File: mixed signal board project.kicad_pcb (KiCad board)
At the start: 4 copper layers, 70.4 x 72.2 mm, 189 parts, among them J101 USB_B_Mini, J102 Conn_01x06_Pin, J201 8P8C_Shielded, J301 Conn_01x04_Pin, J401 AudioJack2_Ground, J402 Conn_01x04_Pin, J403 Screw_Terminal_01x03, J501 USB_B_Mini, J701 Conn_01x02_Socket, J801 Conn_01x02_Socket, J901 UART_CONN, J902 CAN_CONN, SW101 SW_SPDT, SW201 SW_SPDT, SW901 SW_SPDT, U101 STM32F103C8Tx, U11 LD1117S33TR_SOT223, U12 LD1117S18TR_SOT223, U201 DP83826ERHBR, U301 ADS122C04IPW, U401 CS43L22-CNZ, U402 IMP34DT05TR, U501 CH340C, U701 DMHT6016LFJ-13, U702 DRV8701, U801 DMHT6016LFJ-13, U802 DRV8701, U901 STM32F407VGTx, Y201 25Mhz, Y901 8MHz

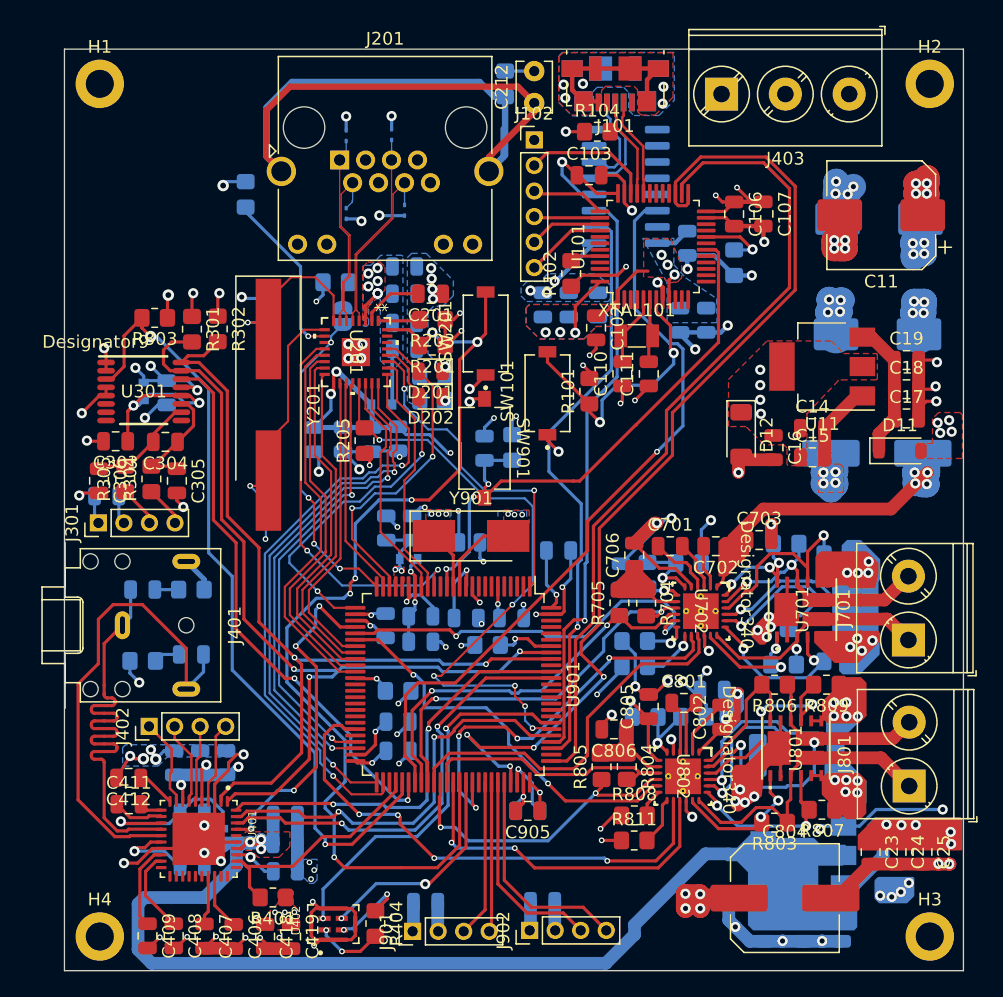
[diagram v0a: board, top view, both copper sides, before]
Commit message: schematic pages are reviewed
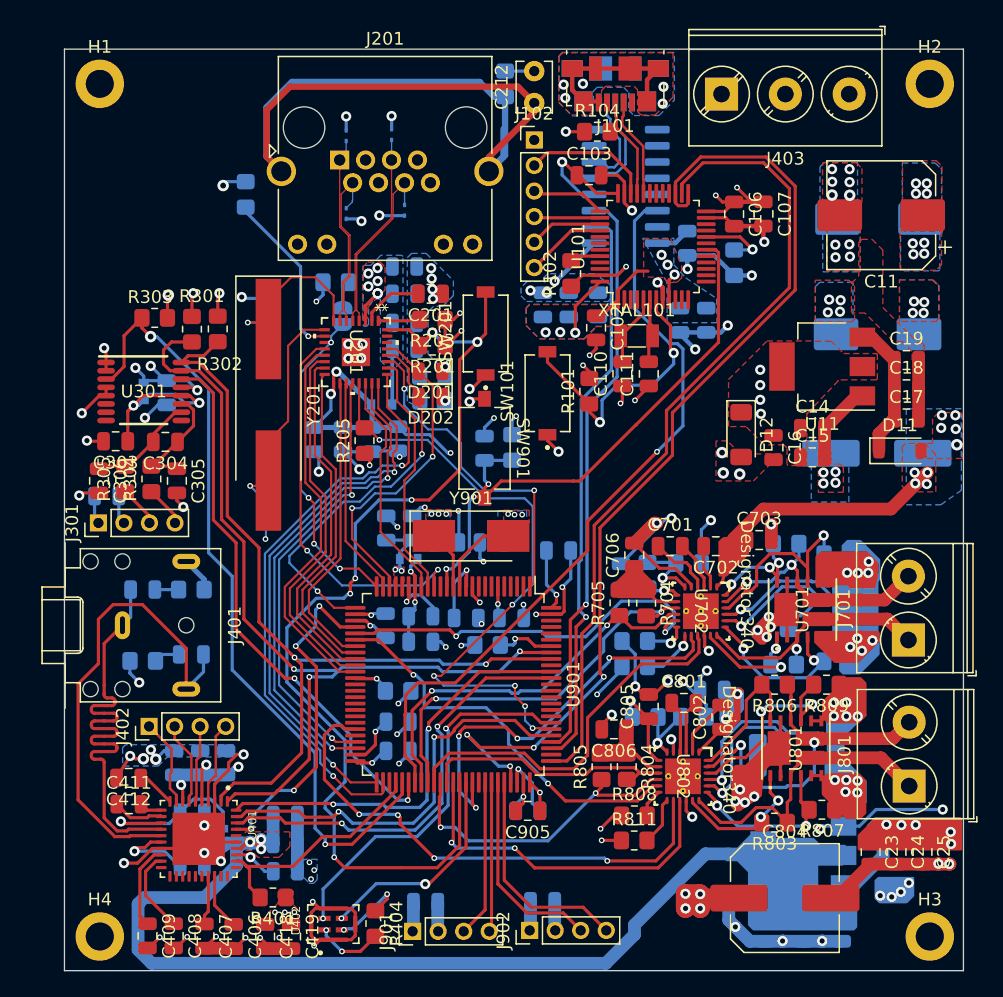
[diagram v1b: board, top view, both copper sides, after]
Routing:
- net GND: track 339.0 -> 305.0 mm, vias 127 -> 128
- net +12V: track 74.7 -> 48.6 mm, vias 38 -> 39
- net /STM32F407/CH340_TXD: track 46.5 -> 44.9 mm
- net /Debugger/JTMS_F407: track 80.0 -> 78.8 mm
- net /STM32F407/CH340_RXD: track 46.1 -> 45.5 mm
- added copper zone on B.Cu, net +12V
